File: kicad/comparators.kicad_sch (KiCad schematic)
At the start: 19 parts

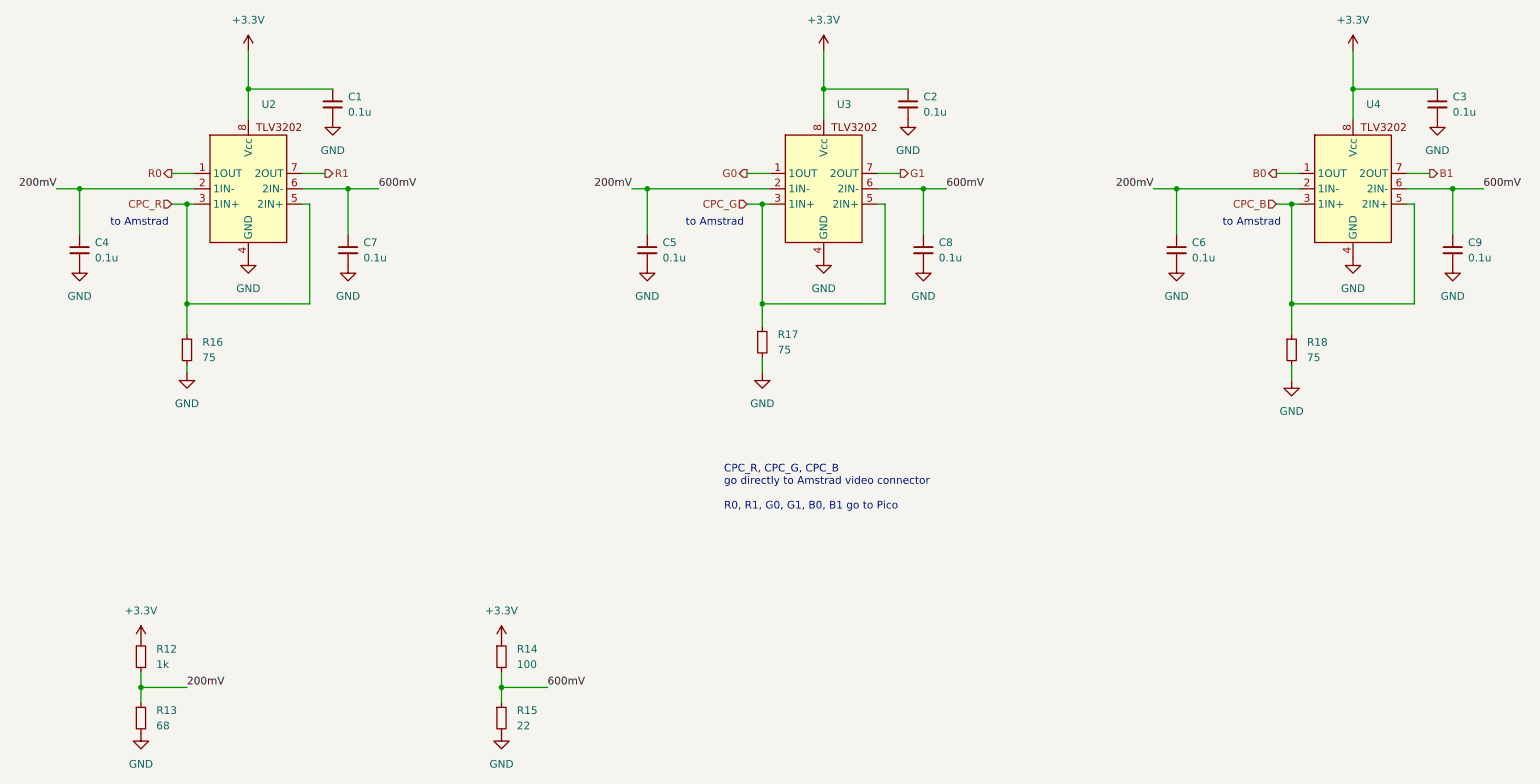
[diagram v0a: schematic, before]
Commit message: Rotated
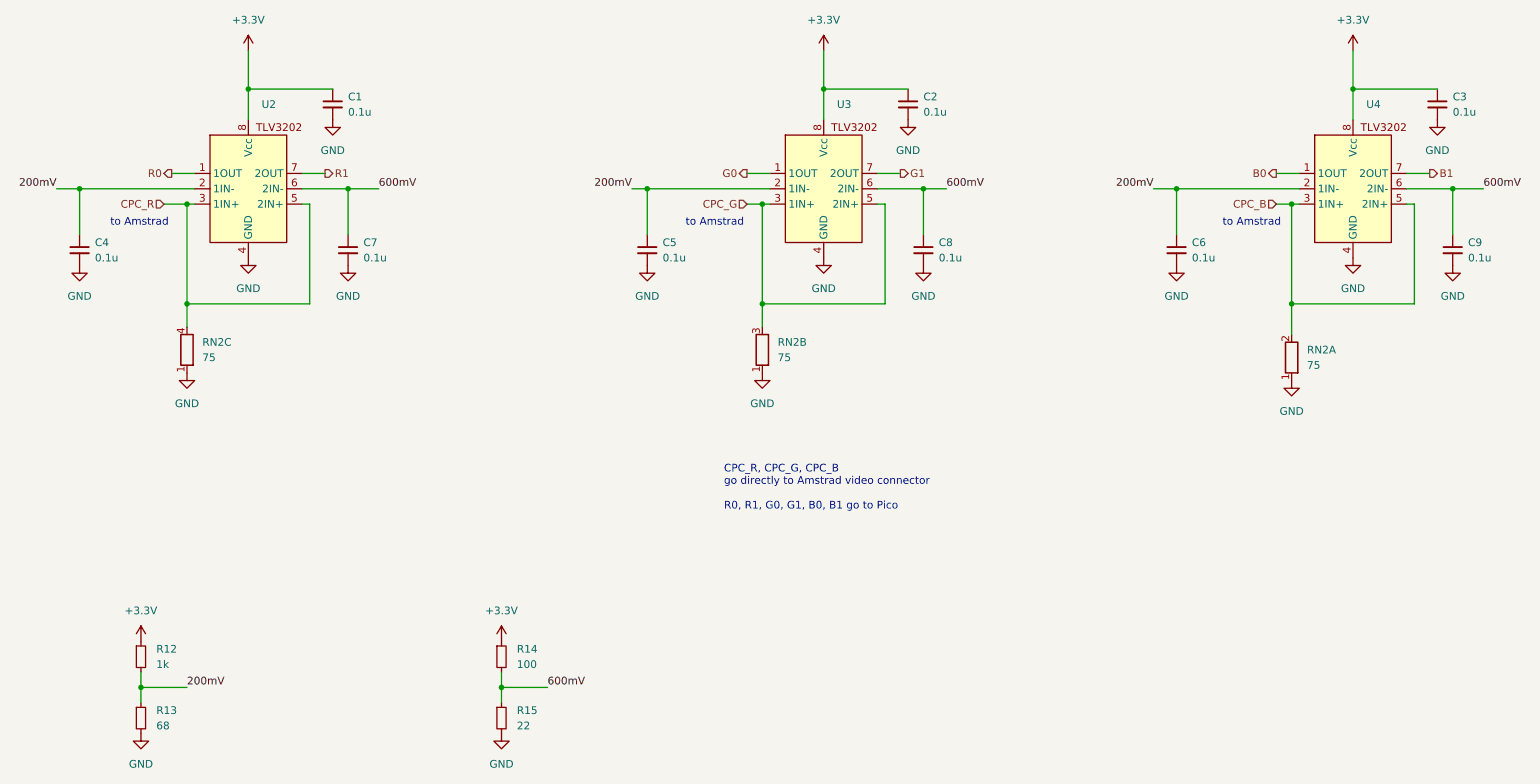
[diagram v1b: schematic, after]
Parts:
- removed R16, R17, R18: 75, Resistor_THT:R_Axial_DIN0207_L6.3mm_D2.5mm_P10.16mm_Horizontal, symbol Device:R_Small
- added RN2: 75, Resistor_THT:R_Array_SIP4, symbol Device:R_Network03_Split
- C1, C2, C3, C4, C5, C6, C7, C8, C9: footprint Capacitor_THT:C_Disc_D4.3mm_W1.9mm_P5.00mm -> Capacitor_SMD:C_1206_3216Metric_Pad1.33x1.80mm_HandSolder
- R12, R13, R14, R15: footprint Resistor_THT:R_Axial_DIN0207_L6.3mm_D2.5mm_P10.16mm_Horizontal -> Resistor_THT:R_Axial_DIN0204_L3.6mm_D1.6mm_P5.08mm_Horizontal
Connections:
- net CPC_B: now also RN2.2 (R1.2)
- net CPC_G: now also RN2.3 (R2.2)
- net CPC_R: now also RN2.4 (R3.2)
- net GND: now also RN2.1 (R1), RN2.1 (R1), RN2.1 (R1)
